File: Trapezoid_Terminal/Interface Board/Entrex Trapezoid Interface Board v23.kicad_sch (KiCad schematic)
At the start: 103 parts, among them P15 Conn_02x40_Odd_Even_Shielded, SW1 SW_DIP_x08

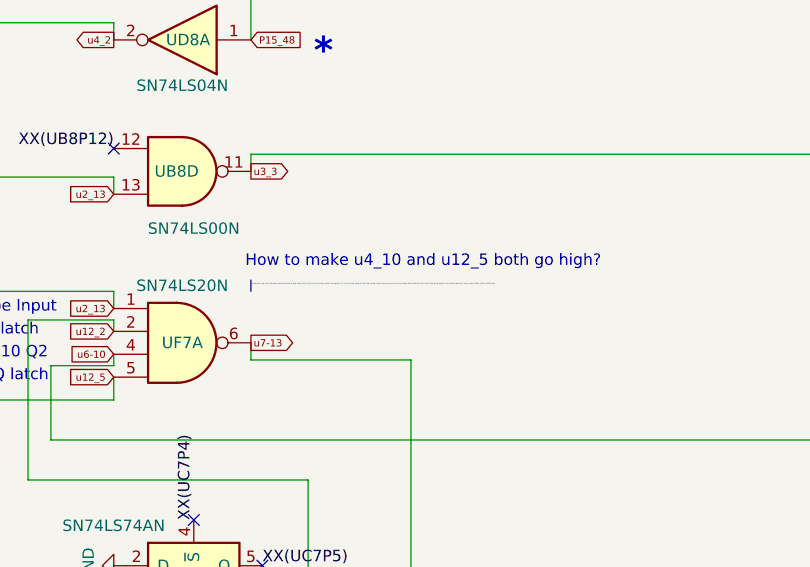
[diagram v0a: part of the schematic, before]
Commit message: talkey
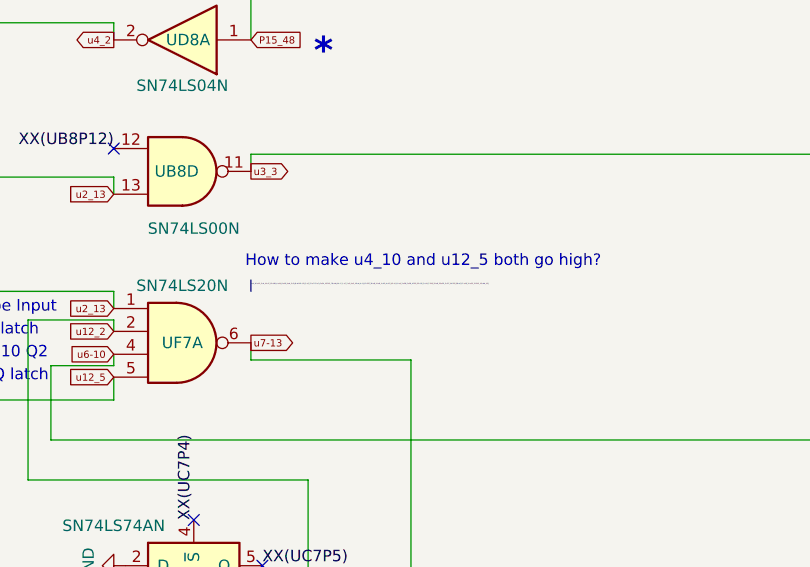
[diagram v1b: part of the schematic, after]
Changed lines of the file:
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@@
     (effects (font (size 1.27 1.27)) (justify left bottom))
   )
-  (label "{u4_10 u12_5 u4_11 u7_10 u28_4 u11_8 u10_9 u4_3 u3_8 u6-10 u12_2 u2_13 u7-13 u7_6 u34_13 P15_79 u44_14 u7_1 u7_5 u3_9 u3_10 u4_4 u3_12 P15_30 u8_11 u9_1 u10_4 u15_12 u2_10 u1_3 u29_5 u29_4 P15_32 u35_3 u11_5 P15_13 u6_13 u20_3 u27_14 P15_28 u6_12 u18_11 u33_12 P15_15 P15_12 P15_23} "
+  (label "{u4_10 u12_5 u4_11 u7_10 u28_4 u11_8 u10_9 u4_3 u3_8 u6-10 u12_2 u2_13 u7-13 u7_6 u34_13 P15_79 u44_14 u7_1 u7_5 u3_9 u3_10 u4_4 u3_12 P15_30 u8_11 u9_1 u10_4 u15_12 u2_10 u1_3 u29_5 u29_4 P15_32 u35_3 u11_5 P15_13 u6_13 u20_3 u27_14 P15_28 u6_12 u18_11 u33_12 P15_15 u44_13}"
     (at 422.91 219.71 0) (fields_autoplaced)
     (effects (font (size 0.125 0.125)) (justify left bottom))
